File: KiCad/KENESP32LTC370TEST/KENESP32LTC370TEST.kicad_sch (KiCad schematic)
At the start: 47 parts, among them J1 Header Pins, Q1 BSC009NE2LS5IATMA1 A (TG2)(1A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, Q2 BSC009NE2LS5IATMA1 B (BG2)(1B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, Q3 BSC009NE2LS5IATMA1 C (BG1)(2A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, Q4 BSC009NE2LS5IATMA1 D (TG1)(2B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, U1 LTC3780EUH-TRPBF

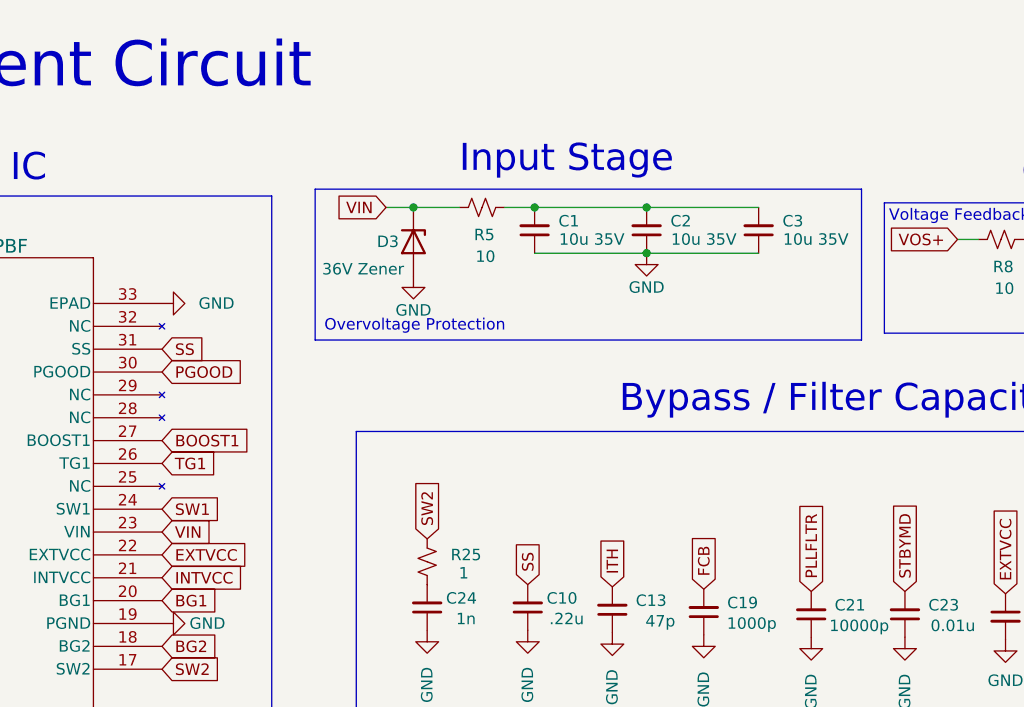
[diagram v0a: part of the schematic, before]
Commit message: PCB Layout Continued
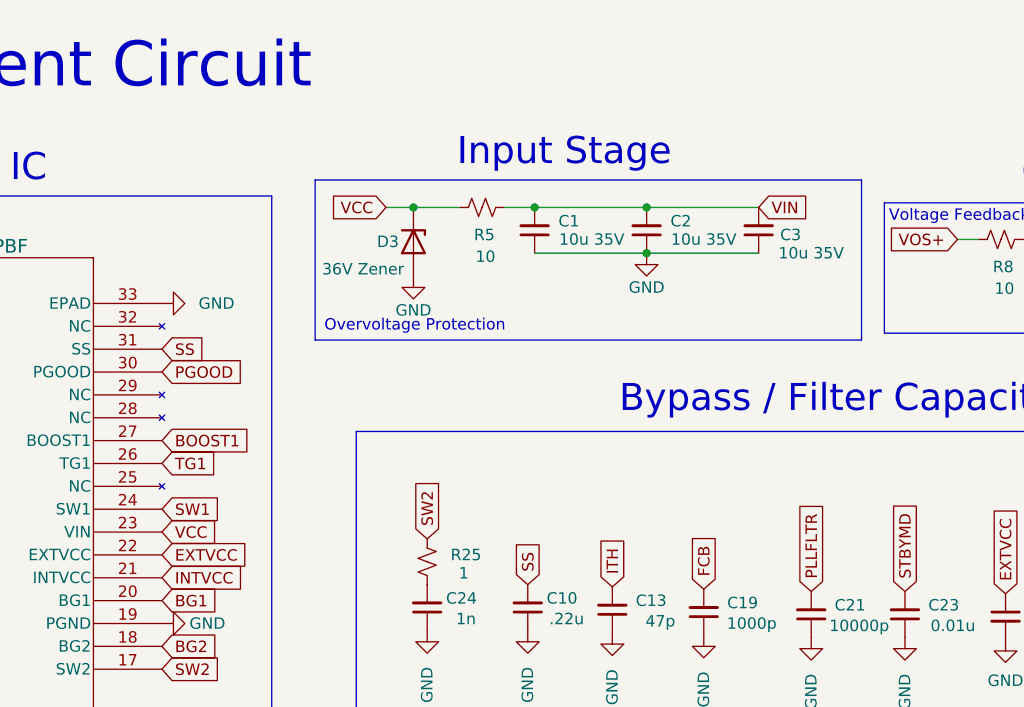
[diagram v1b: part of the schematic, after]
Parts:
- R26: footprint Resistor_SMD:R_1210_3225Metric_Pad1.30x2.65mm_HandSolder -> Resistor_SMD:R_1206_3216Metric_Pad1.30x1.75mm_HandSolder
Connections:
- net VIN: now also C1.2, C2.2, C3.2, R5.1; no longer D3.1 (K), R5.2, U1.23 (VIN)
- new net VCC: D3.1 (K), R5.2, U1.23 (VIN)
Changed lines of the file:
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@@
     (fill (type none))
   )
-  (rectangle (start 244.602 78.994) (end 305.308 95.758)
+  (rectangle (start 244.602 77.978) (end 305.308 95.758)
     (stroke (width 0) (type default))
     (fill (type none))
@@
     (effects (font (size 3 3)) (justify left bottom))
   )
-  (text "Input Stage" (at 260.604 77.47 0)
+  (text "Input Stage" (at 260.35 76.708 0)
     (effects (font (size 3 3)) (justify left bottom))
   )
@@
     )
   )
-  (global_label "VIN" (shape input) (at 227.584 117.094 0) (fields_autoplaced)
-    (effects (font (size 1.27 1.27)) (justify left))
-    (property "Intersheetrefs" "${INTERSHEET_REFS}" (at 233.5137 117.094 0)
-      (effects (font (size 1.27 1.27)) (justify left) hide)
+  (global_label "VCC" (shape input) (at 227.584 117.094 0) (fields_autoplaced)
+    (effects (font (size 1.27 1.27)) (justify left))
+    (property "Intersheetrefs" "${INTERSHEET_REFS}" (at 234.1184 117.094 0)
+      (effects (font (size 1.27 1.27)) (justify left) hide)
+    )
+  )
+  (global_label "VCC" (shape input) (at 252.476 81.026 180) (fields_autoplaced)
+    (effects (font (size 1.27 1.27)) (justify right))
+    (property "Intersheetrefs" "${INTERSHEET_REFS}" (at 245.9416 81.026 0)
+      (effects (font (size 1.27 1.27)) (justify right) hide)
     )
   )
@@
     )
   )
+  (global_label "VIN" (shape input) (at 293.878 81.026 0) (fields_autoplaced)
+    (effects (font (size 1.27 1.27)) (justify left))
+    (property "Intersheetrefs" "${INTERSHEET_REFS}" (at 299.8077 81.026 0)
+      (effects (font (size 1.27 1.27)) (justify left) hide)
+    )
+  )
   (global_label "SW2" (shape input) (at 122.428 185.42 180) (fields_autoplaced)
     (effects (font (size 1.27 1.27)) (justify right))
@@
     (effects (font (size 1.27 1.27)) (justify right))
     (property "Intersheetrefs" "${INTERSHEET_REFS}" (at 307.8692 84.582 0)
-      (effects (font (size 1.27 1.27)) (justify right) hide)
-    )
-  )
-  (global_label "VIN" (shape input) (at 252.476 81.026 180) (fields_autoplaced)
-    (effects (font (size 1.27 1.27)) (justify right))
-    (property "Intersheetrefs" "${INTERSHEET_REFS}" (at 246.5463 81.026 0)
       (effects (font (size 1.27 1.27)) (justify right) hide)
     )
@@
       (effects (font (size 1.27 1.27)))
     )
-    (property "Footprint" "Resistor_SMD:R_1210_3225Metric_Pad1.30x2.65mm_HandSolder" (at 229.108 196.596 0)
+    (property "Footprint" "Resistor_SMD:R_1206_3216Metric_Pad1.30x1.75mm_HandSolder" (at 229.108 196.596 0)
       (effects (font (size 1.27 1.27)) hide)
     )
@@
   (symbol (lib_id "Device:C_Small") (at 293.878 83.566 180) (unit 1)
     (in_bom yes) (on_board yes) (dnp no)
-    (property "Reference" "C3" (at 297.688 82.55 0)
-      (effects (font (size 1.27 1.27)))
-    )
-    (property "Value" "10u 35V" (at 300.228 84.582 0)
-      (effects (font (size 1.27 1.27)))
-    )
+    (property "Reference" "C3" (at 297.434 84.074 0)
+      (effects (font (size 1.27 1.27)))
+    )
+    (property "Value" "10u 35V" (at 299.72 86.106 0)
+      (effects (font (size 1.27 1.27)))
+    )
